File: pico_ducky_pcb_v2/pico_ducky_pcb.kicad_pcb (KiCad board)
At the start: 4 copper layers, 14 x 30 mm, 31 parts, among them J1 USB_A, SW1 R-667799, SW2 R-667799, U1 MIC5504-3.3YMT, U2 W25Q32JVZP, U3 RP2040, Y1 Crystal_GND24

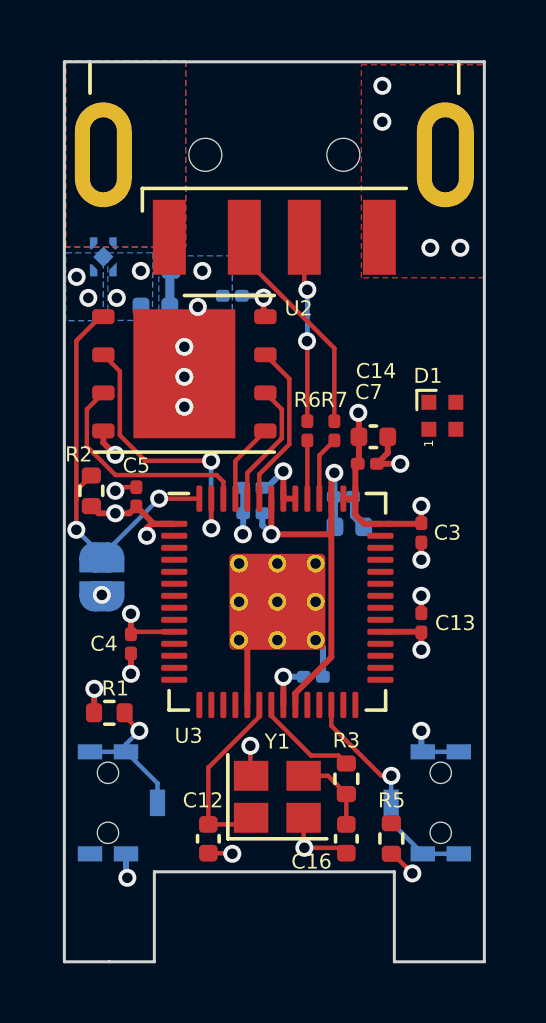
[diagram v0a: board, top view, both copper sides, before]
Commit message: finish routing neopizel
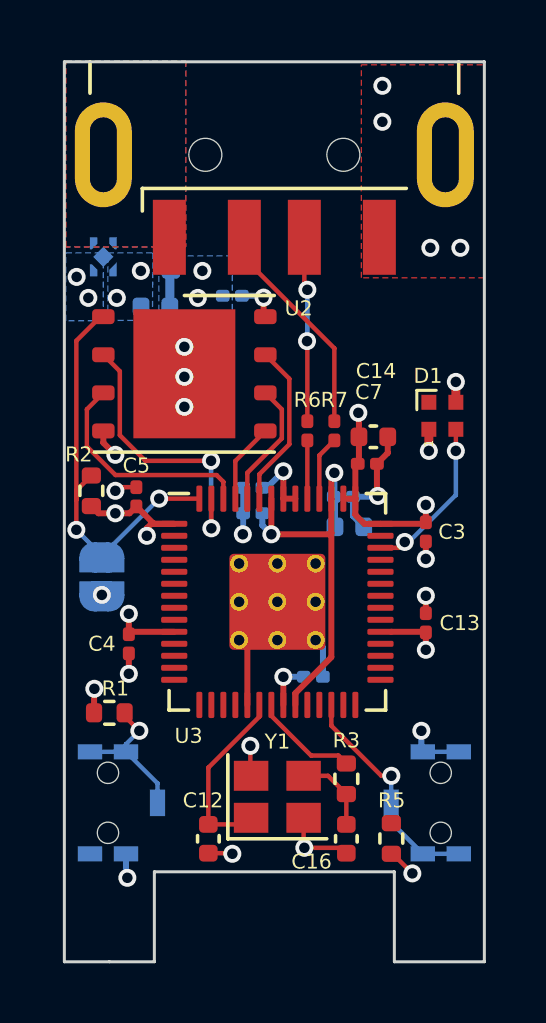
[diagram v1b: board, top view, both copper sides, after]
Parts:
- moved C3 0.15 mm to (92.0, 55.7)
- moved C13 0.15 mm to (92.0, 58.7)
- moved C4 0.07 mm to (82.2, 59.4)
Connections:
- U3 pad 15: /RGB_DI -> unconnected-(U3-Pad15)
- U3 pad 32: /USB_BOOT -> unconnected-(U3-Pad32)
- U3 pad 40: unconnected-(U3-Pad40) -> /RGB_DI
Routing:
- net /RGB_DI: track 0.00 -> 5.43 mm, vias 0 -> 2
- net +3V3: track 22.2 -> 24.7 mm, vias 13 -> 14
- net GND: track 20.0 -> 21.8 mm, vias 24 -> 25
